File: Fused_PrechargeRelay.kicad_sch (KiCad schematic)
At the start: 17 parts, among them K2 DE1a-12V, U5 EL3H7

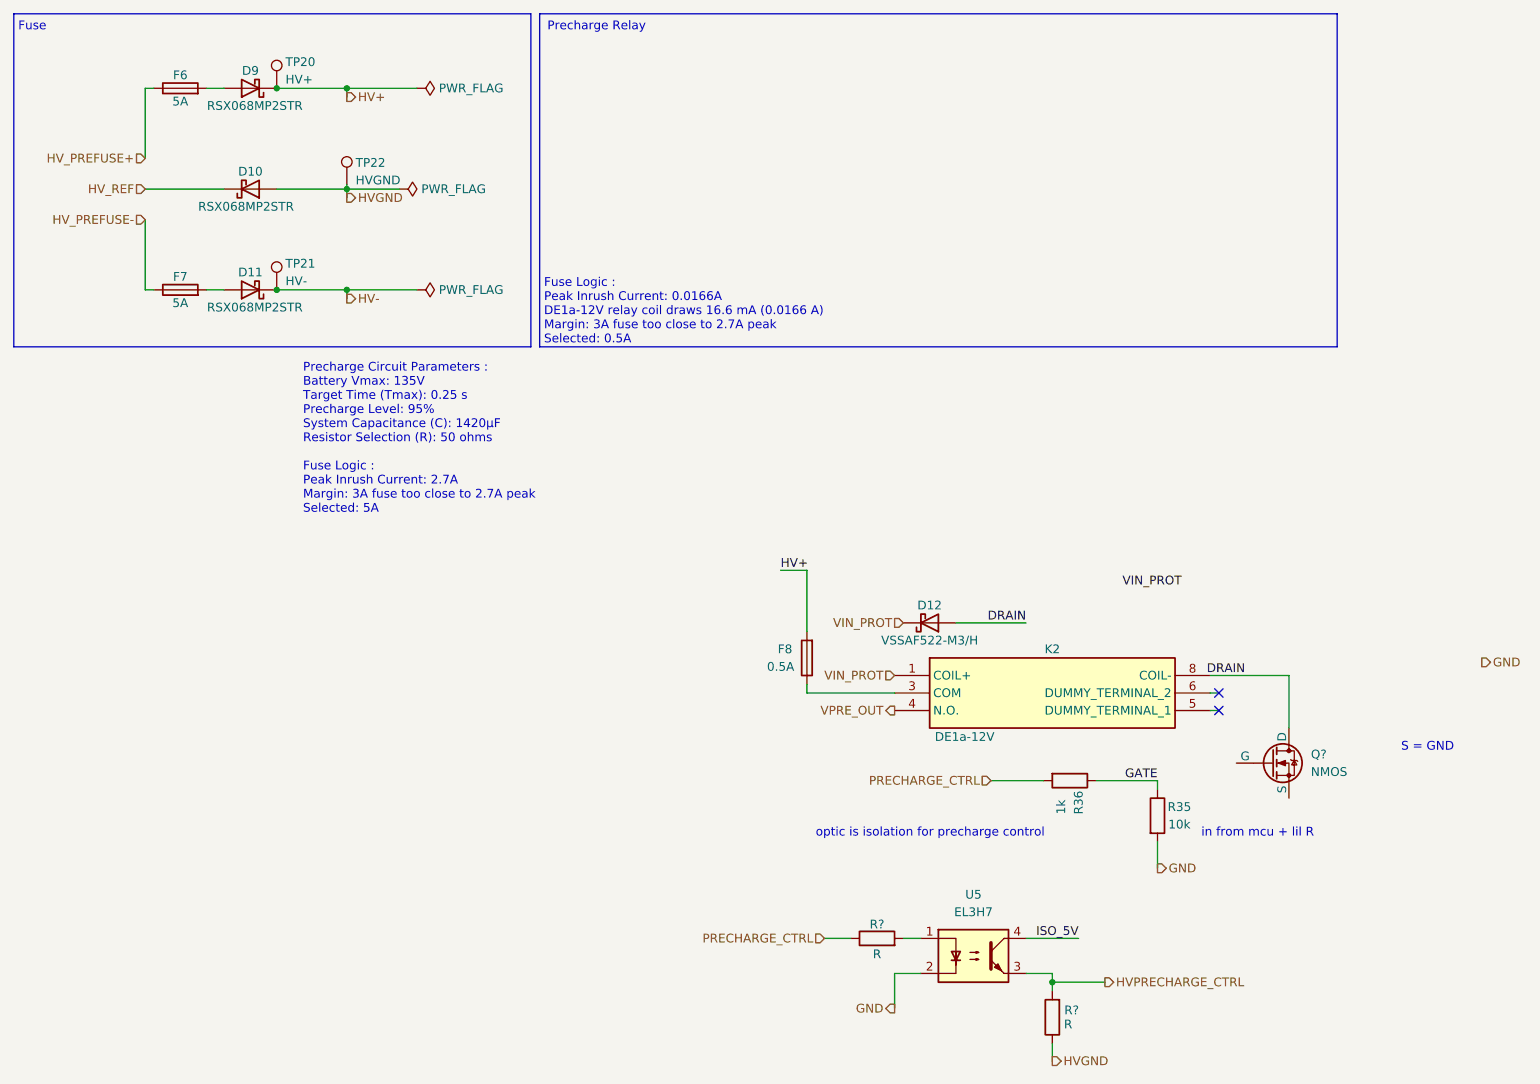
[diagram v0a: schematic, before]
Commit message: final schematic REV-A?
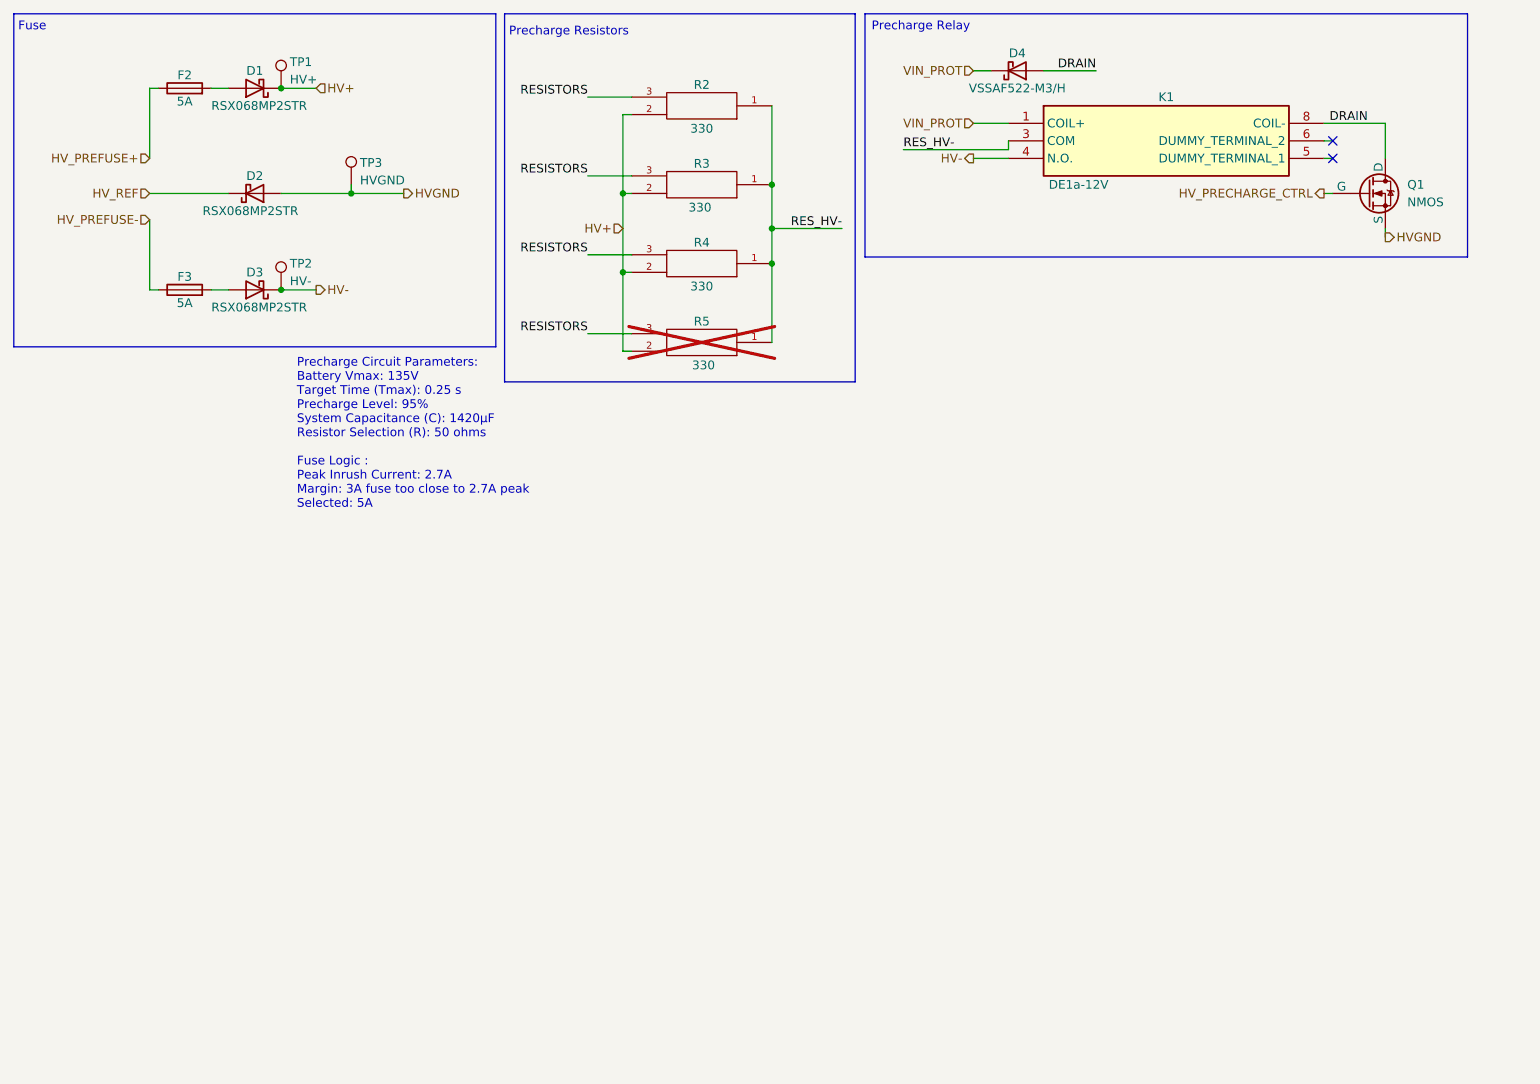
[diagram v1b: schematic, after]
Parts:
- removed F8: 0.5A, symbol Device:Fuse
- removed R35: 10k, Package_DIP:DIP-8_W7.62mm, symbol Device:R
- removed R36: 1k, Package_DIP:DIP-8_W7.62mm, symbol Device:R
- removed R? (x2): R, symbol Device:R
- removed U5: EL3H7, LHRS_ICs:EL3H7, symbol lhrs_ics:EL3H7
- added R2, R3, R4, R5: 330, ActivePrecharge-RevB:RES_PWR263S-35-3300F, symbol Precharge-R:PWR263S-35-3300F
- gave numbers to parts that had none: 1
- renumbered D9 to D1, D10 to D2, D11 to D3, D12 to D4, F6 to F2, F7 to F3, K2 to K1, TP20 to TP1, TP21 to TP2, TP22 to TP3
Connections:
- net VPRE_OUT is gone; now on net HV-: K1.4 (N.O.)
- net HV+: now also R2.2, R3.2, R4.2, R5.2
- net HVGND: now also Q1.3 (S)
- net HV_PRECHARGE_CTRL: now reaches Q1.2 (G)
- net RES_HV-: now reaches K1.3 (COM)
- net RES_HV-: now also R2.1, R3.1, R4.1, R5.1
- new net RESISTORS: R2.3, R3.3, R4.3, R5.3
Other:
- note added: "Precharge Circuit Parameters: Battery Vmax: 135V Target Time (Tmax): 0.25 s Precharge Level: 95% System Capacitance (C): 1420µF Resistor Selection (R): 50 ohms Fuse Logic : Peak Inrush Current: 2.7A Margin: 3A fuse too close to 2.7A peak Selected: 5A"
- note added: "Precharge Resistors"
- note removed: "Fuse Logic : Peak Inrush Current: 0.0166A DE1a-12V relay coil draws 16.6 mA (0.0166 A) Margin: 3A fuse too close to 2.7A peak Selected: 0.5A"
- note removed: "Precharge Circuit Parameters : Battery Vmax: 135V Target Time (Tmax): 0.25 s Precharge Level: 95% System Capacitance (C): 1420µF Resistor Selection (R): 50 ohms Fuse Logic : Peak Inrush Current: 2.7A Margin: 3A fuse too close to 2.7A peak Selected: 5A"
- note removed: "S = GND"
- note removed: "in from mcu + lil R"
- note removed: "optic is isolation for precharge control"
- moved on the sheet: D1, D2, D3, D4, F2, F3, K1, Q1, TP1, TP2, TP3
